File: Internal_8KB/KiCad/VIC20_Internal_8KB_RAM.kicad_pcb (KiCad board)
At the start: 2 copper layers, 70 x 60 mm, 10 parts, among them J1 UD4, J2 UE4, J3 SW, J4 Signals, U1 6264, U2 GAL16V8

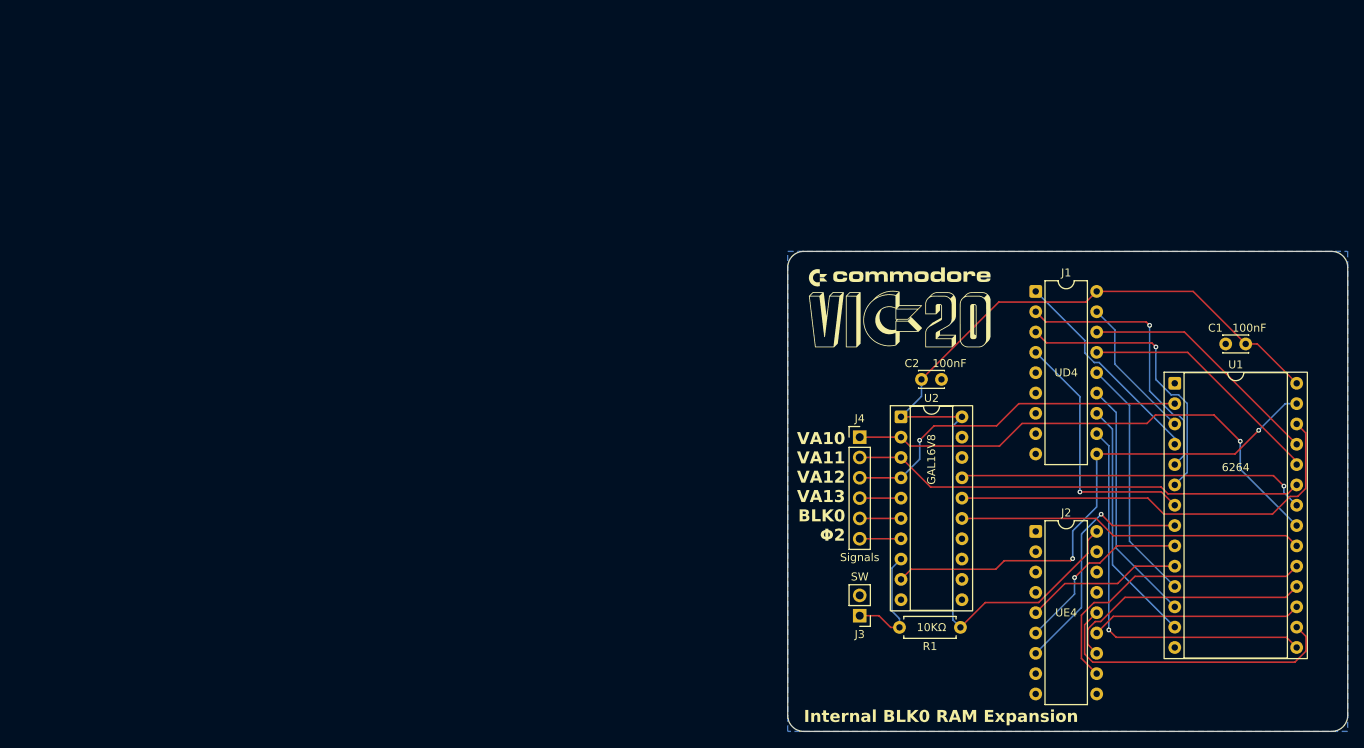
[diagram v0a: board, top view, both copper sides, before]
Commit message: Cosmetic updates to schematic
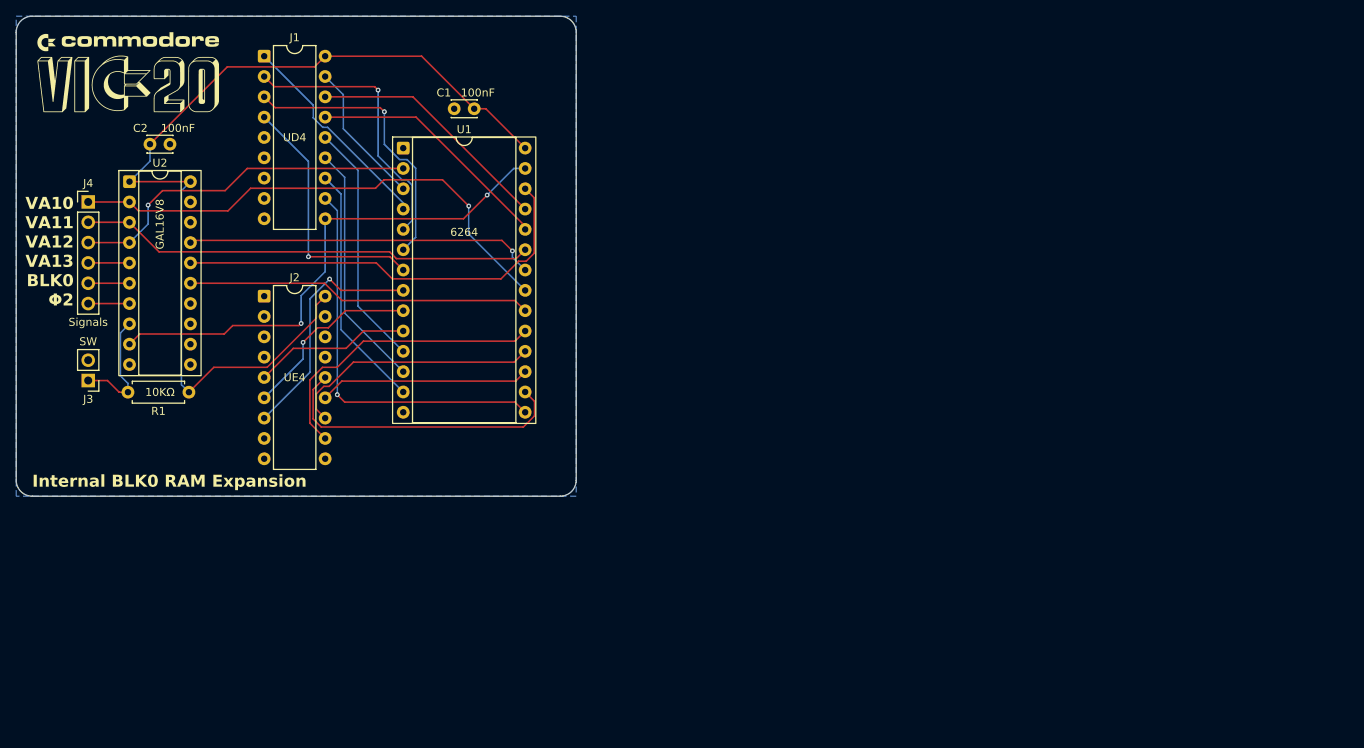
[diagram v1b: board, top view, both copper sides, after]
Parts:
- moved U1 100.8 mm to (97.4, 47.6)
- moved G*** 100.8 mm to (63.0, 38.1)
- moved J3 100.8 mm to (58.0, 76.7)
- moved C1 100.8 mm to (106.3, 42.7)
- moved C2 100.8 mm to (65.8, 47.1)
- moved J1 100.8 mm to (80.0, 36.1)
- moved J2 100.8 mm to (80.0, 66.1)
- moved J4 100.8 mm to (58.0, 54.3)
- moved R1 100.8 mm to (70.6, 78.1)
- moved U2 100.8 mm to (63.2, 51.8)
